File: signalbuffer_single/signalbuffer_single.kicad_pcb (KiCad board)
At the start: 2 copper layers, 35.6 x 17.8 mm, 13 parts, among them J1 GND in, J2 VDD in, J3 VSS in, J4 Signal gnd, J6 Signal In, J7 Bias In, J9 Signal out, U1 LM318N

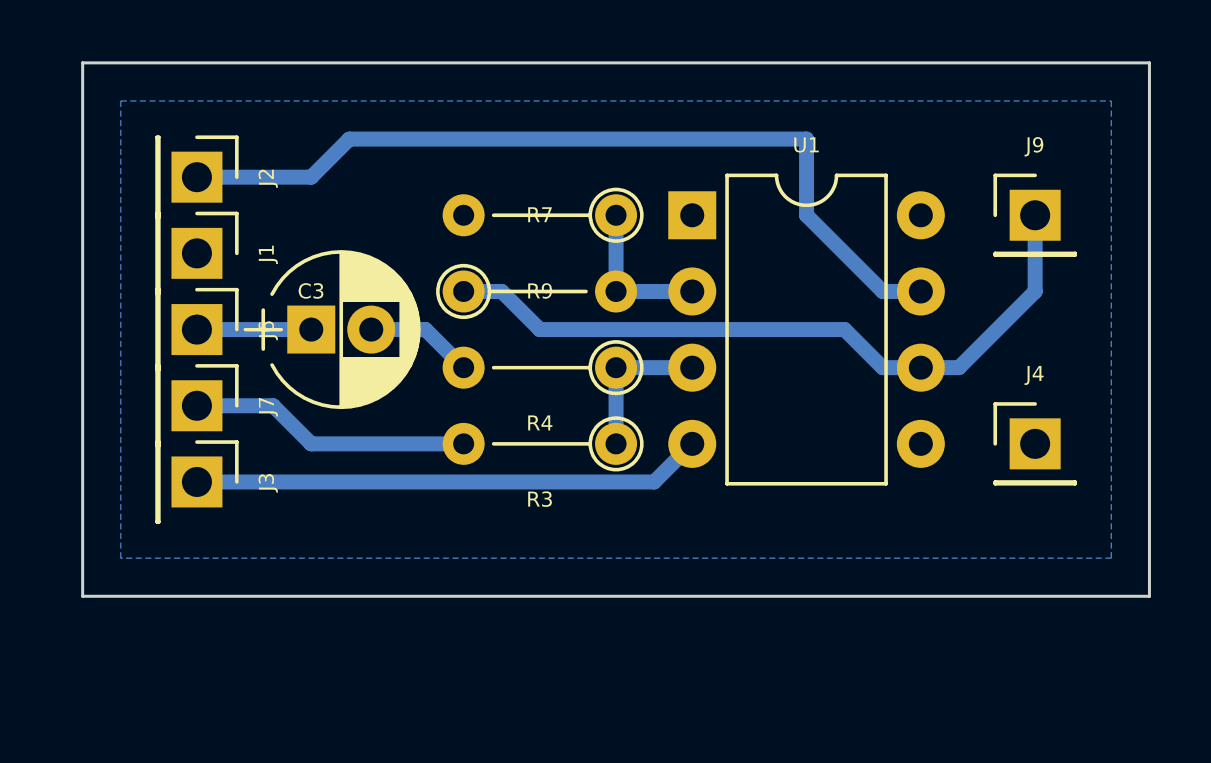
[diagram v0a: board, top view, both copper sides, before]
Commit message: updates
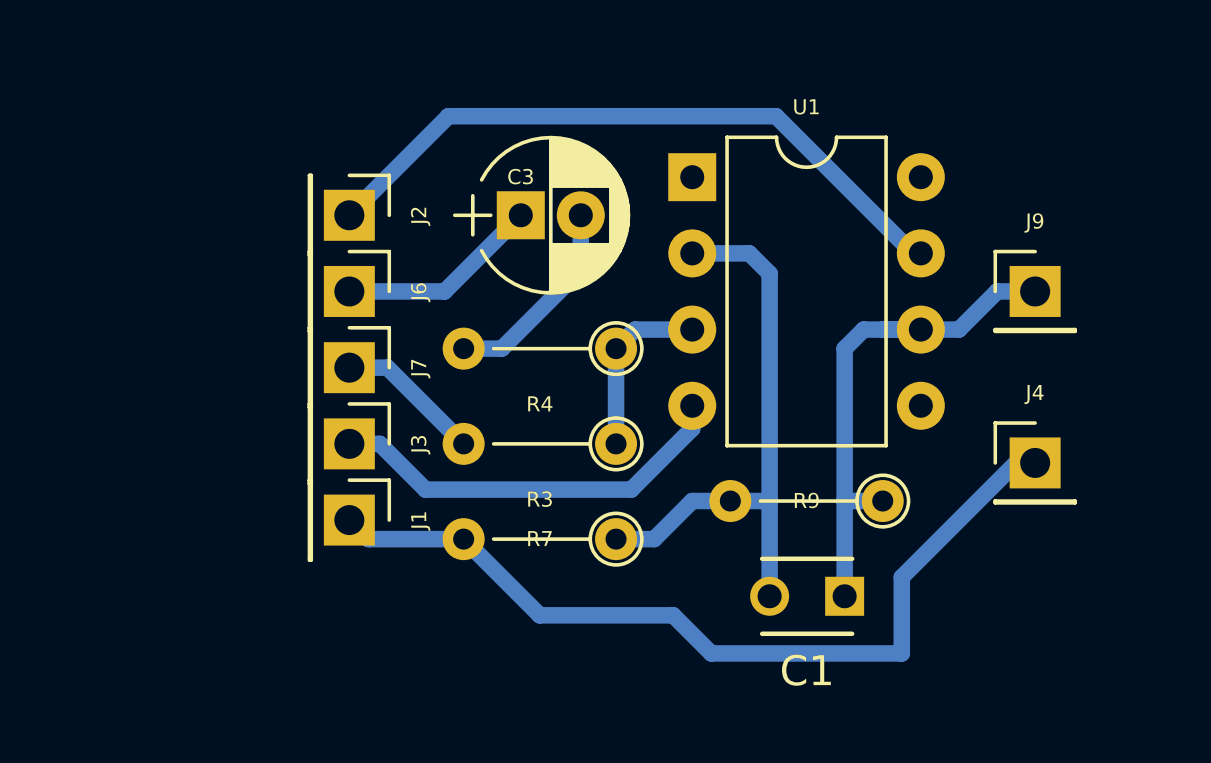
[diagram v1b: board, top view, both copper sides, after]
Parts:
- added C1: C_Small, Capacitors_ThroughHole:C_Disc_D3_P2.5, F.Cu at (160.0, 113.0)
- moved R9 15.6 mm to (161.3, 109.9), turned to 180 degrees
- moved R7 10.8 mm to (152.4, 111.1)
- moved J1 10.2 mm to (143.5, 110.5)
- moved C3 7.96 mm to (149.2, 100.3)
- moved J7 5.24 mm to (143.5, 105.4)
- moved J2 5.24 mm to (143.5, 100.3)
- moved J3 5.24 mm to (143.5, 108.0)
- moved J6 5.24 mm to (143.5, 102.9)
- moved J9 2.54 mm to (166.4, 102.9)
- moved U1 1.27 mm to (154.9, 99.1)
- moved J4 0.63 mm to (166.4, 108.6)
- moved R4 0.63 mm to (152.4, 104.8)
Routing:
- net GNDPWR: track 0.00 -> 28.8 mm
- net Net-(C1-Pad2): track 5.08 -> 19.3 mm
- net Net-(C1-Pad1): track 23.7 -> 17.9 mm
- net Net-(J2-Pad1): track 28.2 -> 22.6 mm
- net Net-(J7-Pad1): track 9.42 -> 4.86 mm
- net Net-(J3-Pad1): track 17.0 -> 13.7 mm
- net Net-(C3-Pad2): track 3.61 -> 6.81 mm
- net Net-(C3-Pad1): track 3.81 -> 6.77 mm
- net Net-(R3-Pad1): track 5.08 -> 5.98 mm
- removed copper zone on B.Cu, net GNDPWR
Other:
- board outline removed
- net class Default: trace_width 0.5 -> 0.55

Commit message: updates
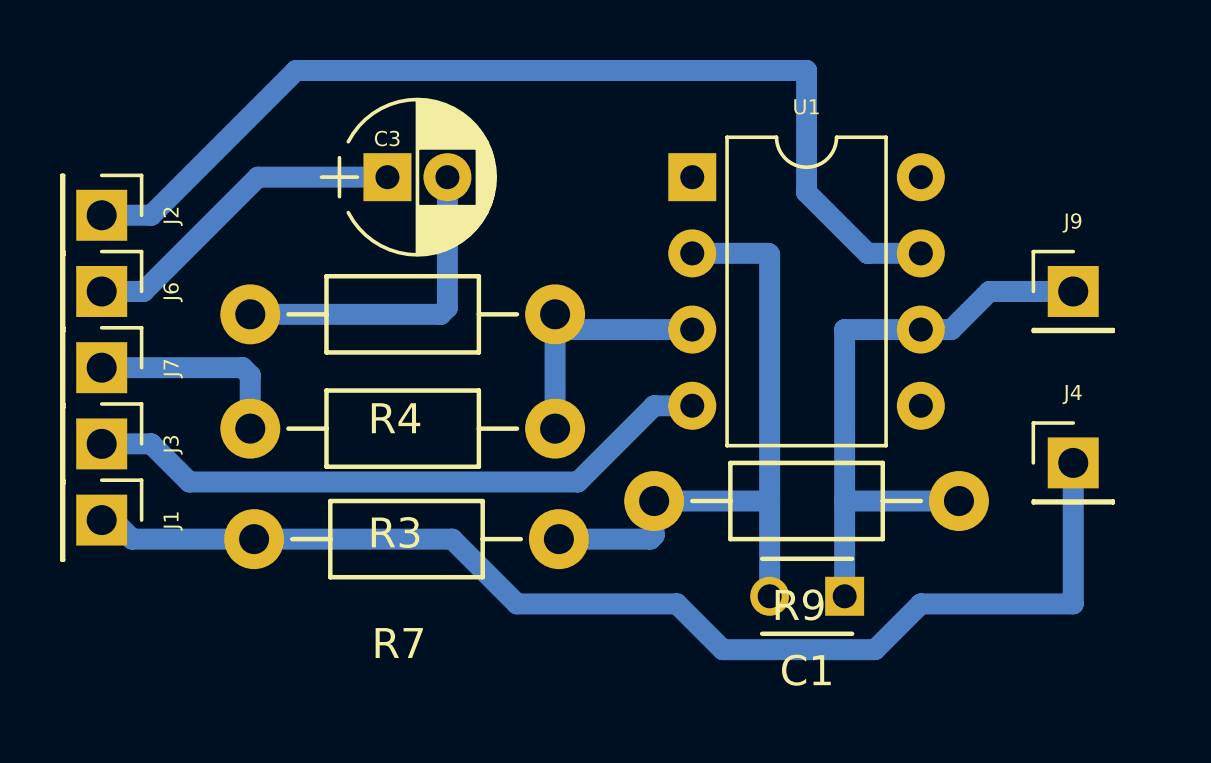
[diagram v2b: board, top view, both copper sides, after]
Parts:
- R3, R4, R7, R9: footprint Resistors_THT:R_Axial_DIN0204_L3.6mm_D1.6mm_P5.08mm_Vertical -> Resistors_ThroughHole:Resistor_Horizontal_RM10mm
- moved J1 8.25 mm to (135.3, 110.5)
- moved J2 8.25 mm to (135.3, 100.3)
- moved J3 8.25 mm to (135.3, 108.0)
- moved J6 8.25 mm to (135.3, 102.9)
- moved J7 8.25 mm to (135.3, 105.4)
- moved C3 4.62 mm to (144.8, 99.1)
- moved R9 2.54 mm to (163.8, 109.9)
- moved R4 2.33 mm to (150.4, 103.6)
- moved R3 2.09 mm to (150.4, 107.4)
- moved R7 1.91 mm to (150.5, 111.1)
- moved J4 1.27 mm to (167.6, 108.6)
- moved J9 1.27 mm to (167.6, 102.9)
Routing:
- net Net-(J2-Pad1): track 22.6 -> 34.5 mm
- net GNDPWR: track 28.8 -> 39.5 mm
- net Net-(J3-Pad1): track 13.7 -> 21.3 mm
- net Net-(C3-Pad1): track 6.77 -> 11.1 mm
- net Net-(C3-Pad2): track 6.81 -> 11.0 mm
- net Net-(C1-Pad1): track 17.9 -> 20.8 mm
- net Net-(C1-Pad2): track 19.3 -> 22.2 mm
- net Net-(R3-Pad1): track 5.98 -> 8.59 mm
- net Net-(J7-Pad1): track 4.86 -> 6.84 mm
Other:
- net class Default: trace_width 0.55 -> 0.7
